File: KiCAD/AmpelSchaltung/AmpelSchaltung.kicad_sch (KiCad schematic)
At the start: 14 parts, among them SW1 SW_DPDT_x2, SW2 SW_DPDT_x2, U1 74HC00, U2 74HC00, U3 AMS1117-3.3

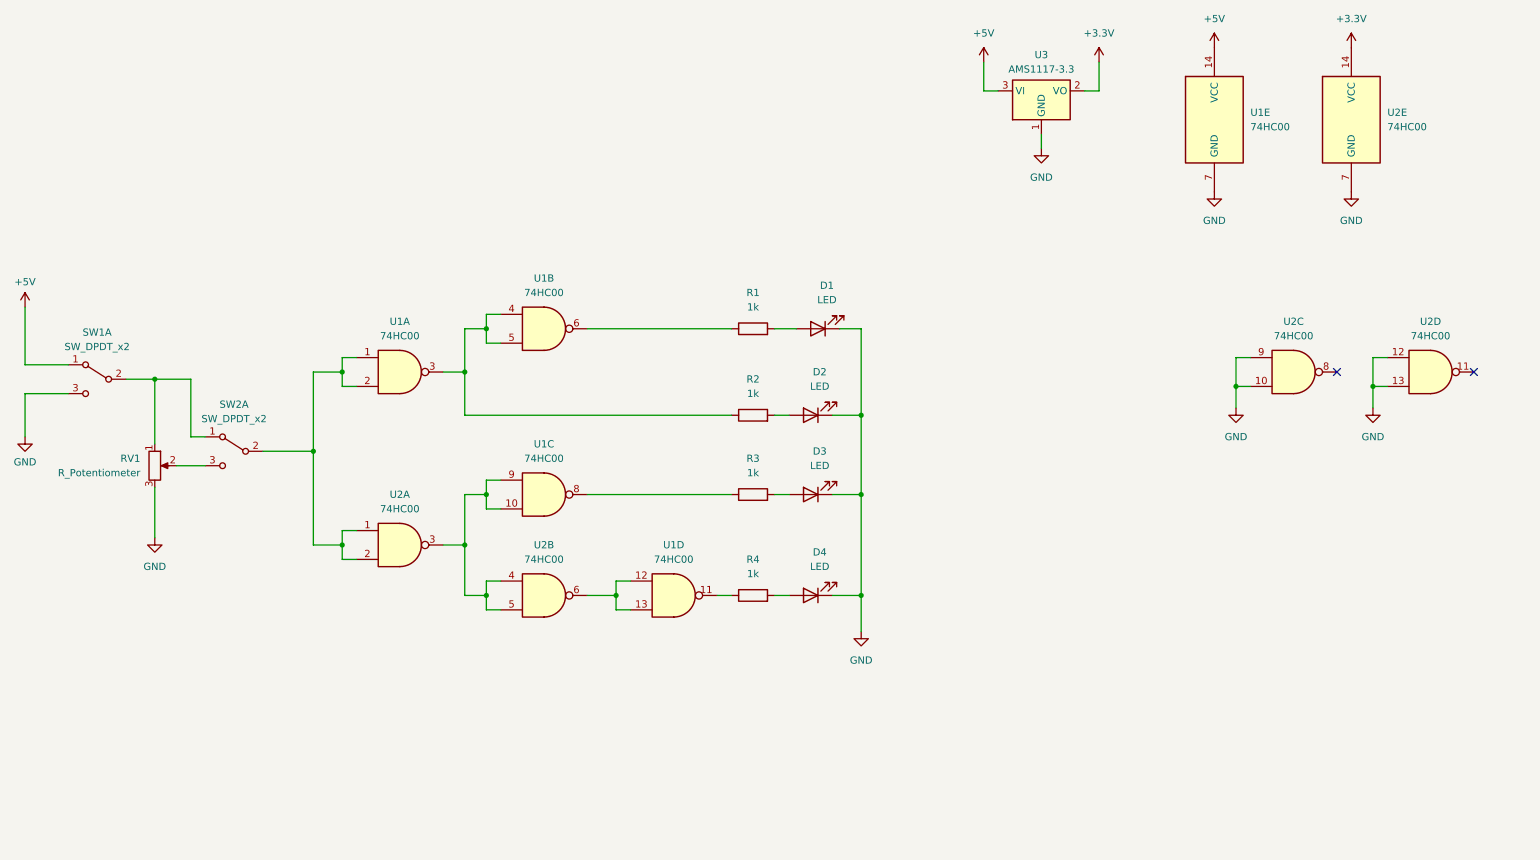
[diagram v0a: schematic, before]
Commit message: update pcb
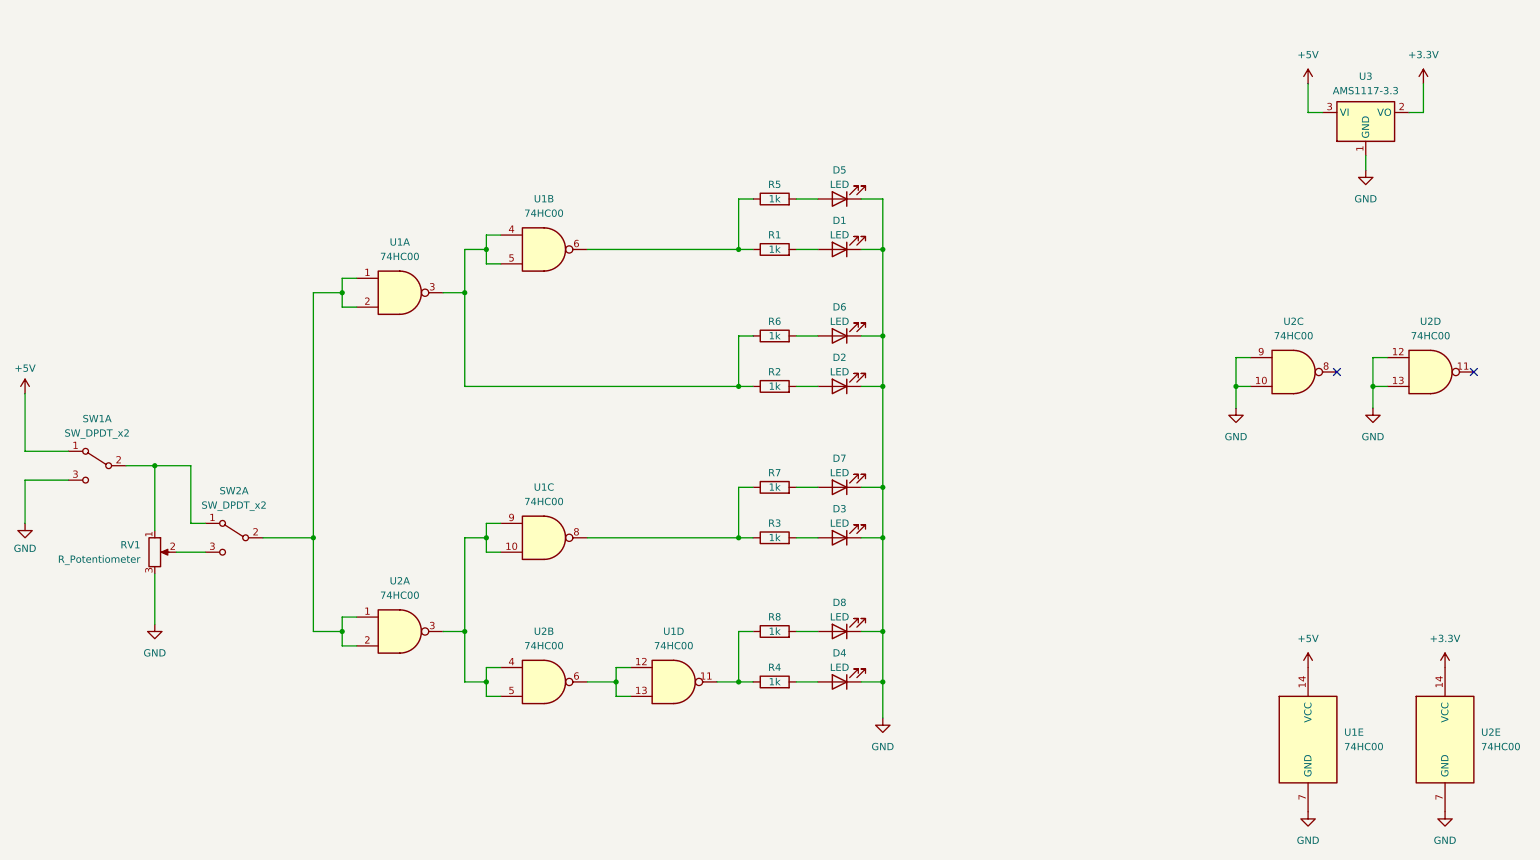
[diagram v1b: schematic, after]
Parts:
- added D5, D6, D7, D8: LED, symbol Device:LED
- added R5, R6, R7, R8: 1k, symbol Device:R
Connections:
- net GND: now also D5.1 (K), D6.1 (K), D7.1 (K), D8.1 (K)
- net at R1.1, U1.6: now also R5.1
- net at R4.1, U1.11: now also R8.1
- net at R2.1, U1.3, U1.4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: now also R6.1
- net at R3.1, U1.8: now also R7.1
- new net: D6.2 (A), R6.2
- new net: D8.2 (A), R8.2
- new net: D7.2 (A), R7.2
- new net: D5.2 (A), R5.2
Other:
- moved on the sheet: D1, D2, D3, D4, R1, R2, R3, R4, RV1, SW1A, SW2A, U1A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
